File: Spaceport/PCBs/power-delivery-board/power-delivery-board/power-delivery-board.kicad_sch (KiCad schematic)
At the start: 61 parts, among them J1 Conn_01x08_Pin, J2 Conn_02x07_Row_Letter_Last, J3 Screw_Terminal_01x02, P1 USB_C_Plug_USB2.0, U1 TPS610986DSER, U2 ADP5033ACBZ-5-R7, U3 TPS610986DSER, U4 LT8609AEDDM-5#TRPBF, U5 USBLC6-2P6, U6 BQ25185DLHR

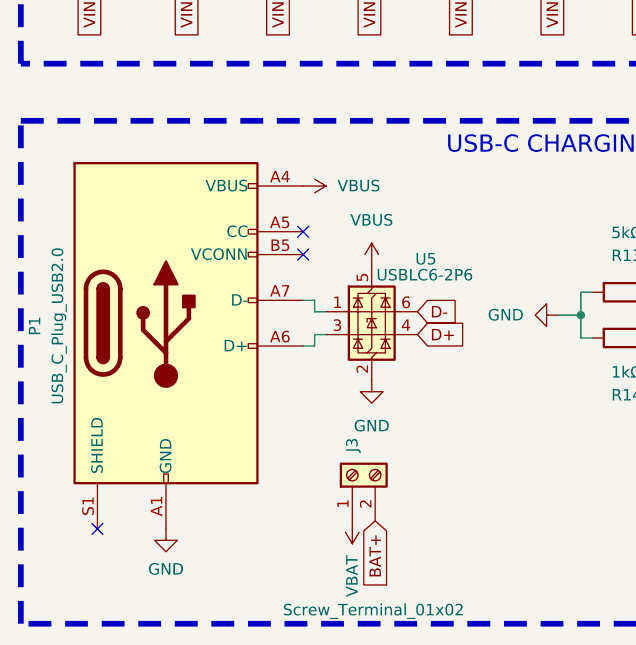
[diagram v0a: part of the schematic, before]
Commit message: Meeting
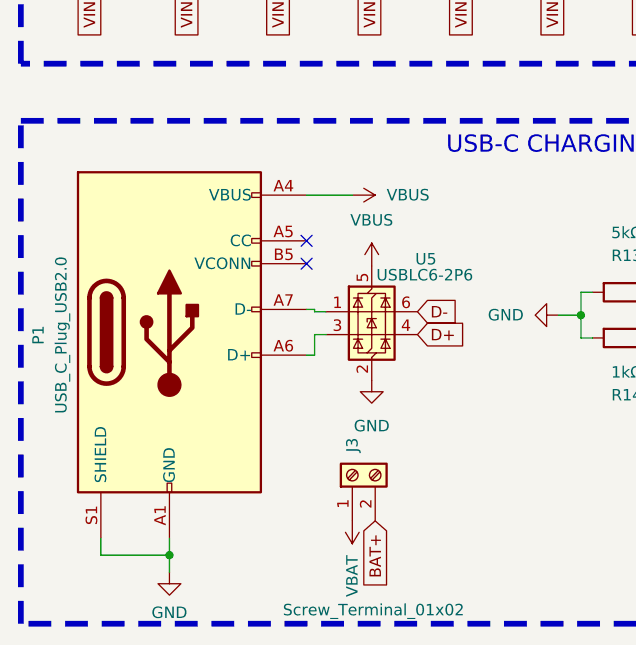
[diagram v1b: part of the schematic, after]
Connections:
- net GND: now also P1.S1 (SHIELD)
- no-connect marks 14 -> 13
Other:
- moved on the sheet: P1
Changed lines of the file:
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@@
 	)
 	(junction
+		(at 29.21 187.96)
+		(diameter 0)
+		(color 0 0 0 0)
+	)
+	(junction
 		(at 50.8 46.99)
 		(diameter 0)
@@
 	)
 	(no_connect
-		(at 21.2073 185.0423)
-	)
-	(no_connect
 		(at 97.79 157.48)
 	)
 	(no_connect
-		(at 44.0673 152.0223)
+		(at 44.45 153.035)
 	)
 	(no_connect
@@
 	)
 	(no_connect
-		(at 44.0673 154.5623)
+		(at 44.45 155.575)
 	)
 	(no_connect
@@
 	(wire
 		(pts
-			(xy 45.3373 164.7223) (xy 45.3373 163.4523)
+			(xy 45.3373 165.735) (xy 45.3373 163.4523)
 		)
 		(stroke
@@
 	(wire
 		(pts
-			(xy 45.3373 159.6423) (xy 45.3373 160.9123)
+			(xy 45.3373 160.655) (xy 45.3373 160.9123)
 		)
 		(stroke
@@
 	(wire
 		(pts
+			(xy 29.21 187.96) (xy 29.21 189.865)
+		)
+		(stroke
+			(width 0)
+			(type default)
+		)
+	)
+	(wire
+		(pts
 			(xy 208.28 34.29) (xy 208.28 39.37)
 		)
@@
 	(wire
 		(pts
-			(xy 44.0673 164.7223) (xy 45.3373 164.7223)
+			(xy 44.45 165.735) (xy 45.3373 165.735)
 		)
 		(stroke
@@
 	(wire
 		(pts
+			(xy 29.21 186.055) (xy 29.21 187.96)
+		)
+		(stroke
+			(width 0)
+			(type default)
+		)
+	)
+	(wire
+		(pts
 			(xy 190.5 123.19) (xy 190.5 140.97)
 		)
@@
 	(wire
 		(pts
+			(xy 44.45 147.955) (xy 49.53 147.955)
+		)
+		(stroke
+			(width 0)
+			(type default)
+		)
+	)
+	(wire
+		(pts
 			(xy 85.09 160.02) (xy 97.79 160.02)
 		)
@@
 	(wire
 		(pts
-			(xy 44.0673 159.6423) (xy 45.3373 159.6423)
+			(xy 44.45 160.655) (xy 45.3373 160.655)
 		)
 		(stroke
@@
 	(wire
 		(pts
+			(xy 21.59 186.055) (xy 21.59 187.96)
+		)
+		(stroke
+			(width 0)
+			(type default)
+		)
+	)
+	(wire
+		(pts
 			(xy 208.28 39.37) (xy 212.09 39.37)
 		)
@@
 	(wire
 		(pts
+			(xy 21.59 187.96) (xy 29.21 187.96)
+		)
+		(stroke
+			(width 0)
+			(type default)
+		)
+	)
+	(wire
+		(pts
 			(xy 209.55 130.81) (xy 209.55 140.97)
 		)
@@
 	)
 	(symbol
+		(lib_id "power:GND")
+		(at 29.21 189.865 0)
+		(unit 1)
+		(exclude_from_sim no)
+		(in_bom yes)
+		(on_board yes)
+		(dnp no)
+		(fields_autoplaced yes)
+		(property "Reference" "#PWR036"
+			(at 29.21 196.215 0)
+			(effects
+				(font
+					(size 1.27 1.27)
+				)
+				(hide yes)
+			)
+		)
+		(property "Value" "GND"
+			(at 29.21 194.3548 0)
+			(effects
+				(font
+					(size 1.27 1.27)
+				)
+			)
+		)
+		(property "Footprint" ""
+			(at 29.21 189.865 0)
+			(effects
+				(font
+					(size 1.27 1.27)
+				)
+				(hide yes)
+			)
+		)
+		(property "Datasheet" ""
+			(at 29.21 189.865 0)
+			(effects
+				(font
+					(size 1.27 1.27)
+				)
+				(hide yes)
+			)
+		)
+		(property "Description" "Power symbol creates a global label with name \"GND\" , ground"
+			(at 29.21 189.865 0)
+			(effects
+				(font
+					(size 1.27 1.27)
+				)
+				(hide yes)
+			)
+		)
+		(pin "1"
+		)
+		(instances
+			(project "power-delivery-board"
+				(path "/ede041fa-5c95-4d07-be56-df14cd7dcdb2"
+					(reference "#PWR036")
+					(unit 1)
+				)
+			)
+		)
+	)
+	(symbol
 		(lib_id "Device:C")
 		(at 256.54 129.54 0)
@@
 	(symbol
 		(lib_id "Connector:USB_C_Plug_USB2.0")
-		(at 28.8273 162.1823 0)
+		(at 29.21 163.195 0)
 		(unit 1)
 		(exclude_from_sim no)
@@
 		(dnp no)
 		(property "Reference" "P1"
-			(at 14.2669 162.4953 90)
+			(at 14.6496 163.508 90)
 			(effects
 				(font
@@
 		)
 		(property "Value" "USB_C_Plug_USB2.0"
-			(at 16.8069 162.4953 90)
+			(at 17.1896 163.508 90)
 			(effects
 				(font
@@
 		)
 		(property "Footprint" "Inductor_SMD:L_0805_2012Metric"
-			(at 32.6373 162.1823 0)
+			(at 33.02 163.195 0)
 			(effects
 				(font
@@
 		)
 		(property "Datasheet" "https://www.usb.org/sites/default/files/documents/usb_type-c.zip"
-			(at 32.6373 162.1823 0)
+			(at 33.02 163.195 0)
 			(effects
 				(font
@@
 		)
 		(property "Description" "USB 2.0-only Type-C Plug connector"
-			(at 28.8273 162.1823 0)
+			(at 29.21 163.195 0)
 			(effects
 				(font
@@
 	)
 	(symbol
-		(lib_id "power:VBUS")
-		(at 44.0673 146.9423 270)
+		(lib_id "Device:L")
+		(at 195.58 123.19 90)
 		(unit 1)
 		(exclude_from_sim no)
@@
 		(dnp no)
 		(fields_autoplaced yes)
-		(property "Reference" "#PWR026"
-			(at 40.2573 146.9423 0)
+		(property "Reference" "L5"
+			(at 195.58 118.11 90)
 			(effects
 				(font
 					(size 1.27 1.27)
 				)
-				(hide yes)
 			)
 		)
-		(property "Value" "VBUS"
-			(at 47.8773 146.9422 90)
+		(property "Value" "2.2uH"
+			(at 195.58 120.65 90)
 			(effects
 				(font
 					(size 1.27 1.27)
 				)
-				(justify left)
 			)
 		)
-		(property "Footprint" ""
-			(at 44.0673 146.9423 0)
+		(property "Footprint" "Inductor_SMD:L_0805_2012Metric"
+			(at 195.58 123.19 0)
 			(effects
 				(font
@@
 			)
 		)
-		(property "Datasheet" ""
-			(at 44.0673 146.9423 0)
+		(property "Datasheet" "~"
+			(at 195.58 123.19 0)
 			(effects
 				(font
@@
 			)
 		)
-		(property "Description" "Power symbol creates a global label with name \"VBUS\""
-			(at 44.0673 146.9423 0)
+		(property "Description" "Inductor"
+			(at 195.58 123.19 0)
 			(effects
 				(font
@@
 			)
 		)
+		(pin "2"
+		)
 		(pin "1"
 		)
@@
 			(project ""
 				(path "/ede041fa-5c95-4d07-be56-df14cd7dcdb2"
-					(reference "#PWR026")
+					(reference "L5")
 					(unit 1)
 				)
@@
 	)
 	(symbol
-		(lib_id "Device:L")
-		(at 195.58 123.19 90)
+		(lib_id "power:VBUS")
+		(at 49.53 147.955 270)
 		(unit 1)
 		(exclude_from_sim no)
@@
 		(dnp no)
 		(fields_autoplaced yes)
-		(property "Reference" "L5"
-			(at 195.58 118.11 90)
+		(property "Reference" "#PWR026"
+			(at 45.72 147.955 0)
 			(effects
 				(font
 					(size 1.27 1.27)
 				)
+				(hide yes)
 			)
 		)
-		(property "Value" "2.2uH"
-			(at 195.58 120.65 90)
+		(property "Value" "VBUS"
+			(at 53.34 147.9549 90)
 			(effects
 				(font
 					(size 1.27 1.27)
 				)
+				(justify left)
 			)
 		)
-		(property "Footprint" "Inductor_SMD:L_0805_2012Metric"
-			(at 195.58 123.19 0)
+		(property "Footprint" ""
+			(at 49.53 147.955 0)
 			(effects
 				(font
@@
 			)
 		)
-		(property "Datasheet" "~"
-			(at 195.58 123.19 0)
+		(property "Datasheet" ""
+			(at 49.53 147.955 0)
 			(effects
 				(font
@@
 			)
 		)
-		(property "Description" "Inductor"
-			(at 195.58 123.19 0)
+		(property "Description" "Power symbol creates a global label with name \"VBUS\""
+			(at 49.53 147.955 0)
 			(effects
 				(font
@@
 			)
 		)
-		(pin "2"
-		)
 		(pin "1"
 		)
 		(instances
-			(project ""
+			(project "power-delivery-board"
 				(path "/ede041fa-5c95-4d07-be56-df14cd7dcdb2"
-					(reference "L5")
+					(reference "#PWR026")
 					(unit 1)
 				)
@@
 					(unit 1)
 				)
-			)
-		)
-	)
-	(symbol
-		(lib_id "power:GND")
-		(at 28.8273 185.0423 0)
-		(unit 1)
-		(exclude_from_sim no)
-		(in_bom yes)
-		(on_board yes)
-		(dnp no)
-		(fields_autoplaced yes)
-		(property "Reference" "#PWR036"
-			(at 28.8273 191.3923 0)
-			(effects
-				(font
-					(size 1.27 1.27)
-				)
-				(hide yes)
-			)
-		)
-		(property "Value" "GND"
-			(at 28.8273 189.5321 0)
-			(effects
-				(font
-					(size 1.27 1.27)
-				)
-			)
-		)
-		(property "Footprint" ""
-			(at 28.8273 185.0423 0)
-			(effects
-				(font
-					(size 1.27 1.27)
-				)
-				(hide yes)
-			)
-		)
-		(property "Datasheet" ""
-			(at 28.8273 185.0423 0)
-			(effects
-				(font
-					(size 1.27 1.27)
-				)
-				(hide yes)
-			)
-		)
-		(property "Description" "Power symbol creates a global label with name \"GND\" , ground"
-			(at 28.8273 185.0423 0)
-			(effects
-				(font
-					(size 1.27 1.27)
-				)
-				(hide yes)
-			)
-		)
-		(pin "1"
-		)
-		(instances
-			(project ""
-				(path "/ede041fa-5c95-4d07-be56-df14cd7dcdb2"
-					(reference "#PWR036")
-					(unit 1)
-				)
